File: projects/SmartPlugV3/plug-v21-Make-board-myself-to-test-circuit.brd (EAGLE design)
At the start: 63.5 x 70 mm, 34 parts

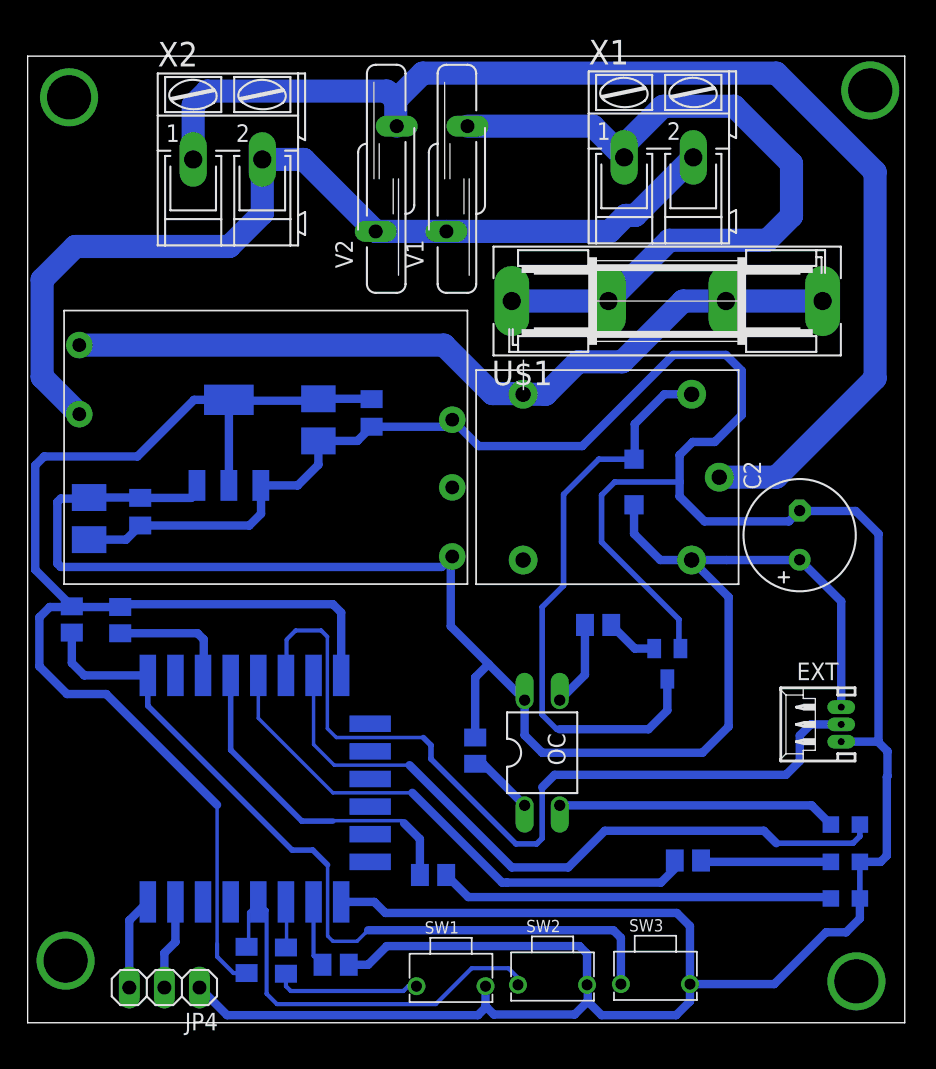
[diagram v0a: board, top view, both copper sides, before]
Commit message: commit message
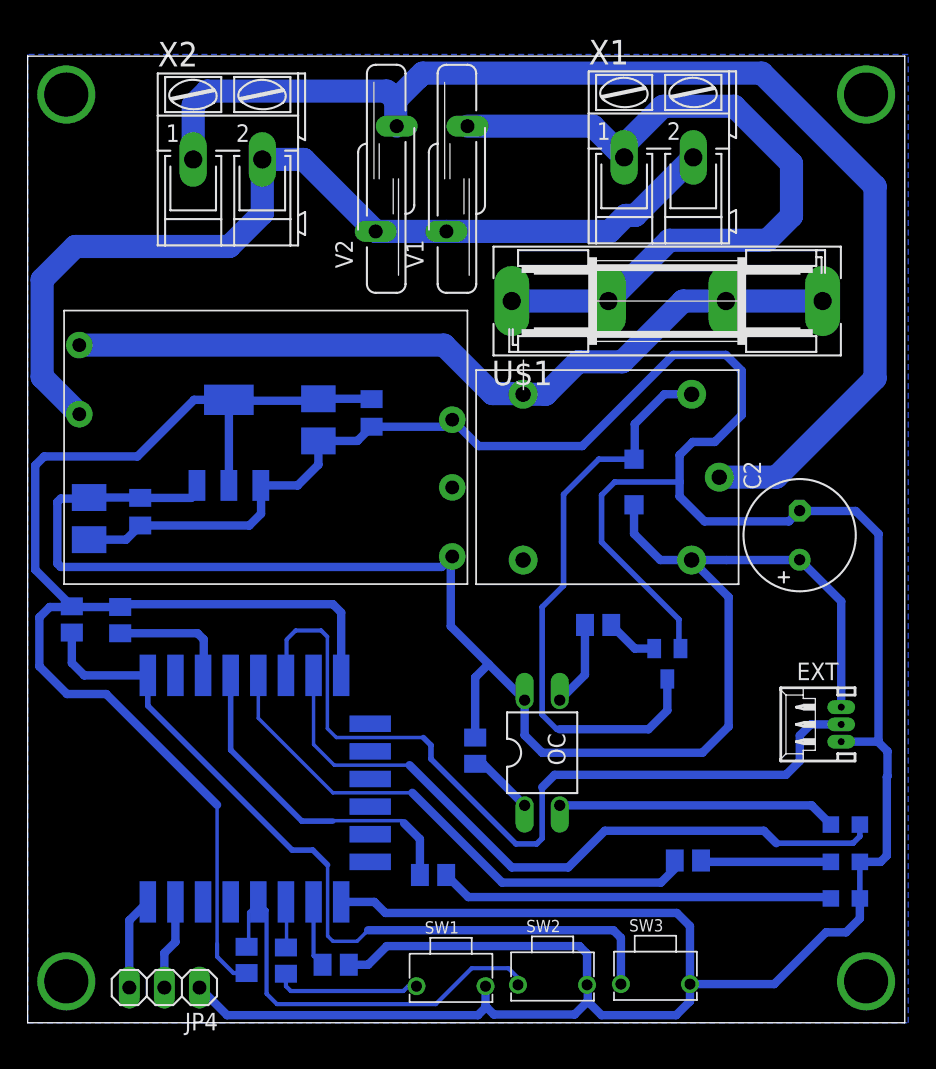
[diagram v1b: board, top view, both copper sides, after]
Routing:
- net RELAY-COM: track 88.9 -> 88.3 mm
- added copper zone on layer 16, net GND
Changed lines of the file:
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@@
 <layer number="37" name="tTest" color="7" fill="1" visible="no" active="yes"/>
 <layer number="38" name="bTest" color="7" fill="1" visible="no" active="yes"/>
-<layer number="39" name="tKeepout" color="4" fill="11" visible="no" active="yes"/>
-<layer number="40" name="bKeepout" color="1" fill="11" visible="no" active="yes"/>
-<layer number="41" name="tRestrict" color="4" fill="10" visible="no" active="yes"/>
-<layer number="42" name="bRestrict" color="1" fill="10" visible="no" active="yes"/>
-<layer number="43" name="vRestrict" color="2" fill="10" visible="no" active="yes"/>
+<layer number="39" name="tKeepout" color="4" fill="11" visible="yes" active="yes"/>
+<layer number="40" name="bKeepout" color="1" fill="11" visible="yes" active="yes"/>
+<layer number="41" name="tRestrict" color="4" fill="10" visible="yes" active="yes"/>
+<layer number="42" name="bRestrict" color="1" fill="10" visible="yes" active="yes"/>
+<layer number="43" name="vRestrict" color="2" fill="10" visible="yes" active="yes"/>
 <layer number="44" name="Drills" color="7" fill="1" visible="no" active="yes"/>
-<layer number="45" name="Holes" color="7" fill="1" visible="no" active="yes"/>
-<layer number="46" name="Milling" color="3" fill="1" visible="no" active="yes"/>
-<layer number="47" name="Measures" color="7" fill="1" visible="no" active="yes"/>
-<layer number="48" name="Document" color="7" fill="1" visible="no" active="yes"/>
-<layer number="49" name="Reference" color="7" fill="1" visible="no" active="yes"/>
+<layer number="45" name="Holes" color="7" fill="1" visible="yes" active="yes"/>
+<layer number="46" name="Milling" color="3" fill="1" visible="yes" active="yes"/>
+<layer number="47" name="Measures" color="7" fill="1" visible="yes" active="yes"/>
+<layer number="48" name="Document" color="7" fill="1" visible="yes" active="yes"/>
+<layer number="49" name="Reference" color="7" fill="1" visible="yes" active="yes"/>
 <layer number="50" name="dxf" color="7" fill="1" visible="no" active="no"/>
-<layer number="51" name="tDocu" color="7" fill="1" visible="no" active="yes"/>
-<layer number="52" name="bDocu" color="7" fill="1" visible="no" active="yes"/>
+<layer number="51" name="tDocu" color="7" fill="1" visible="yes" active="yes"/>
+<layer number="52" name="bDocu" color="7" fill="1" visible="yes" active="yes"/>
 <layer number="53" name="tGND_GNDA" color="7" fill="9" visible="no" active="no"/>
 <layer number="54" name="bGND_GNDA" color="1" fill="9" visible="no" active="no"/>
@@
 <wire x1="62.25" y1="17.85" x2="62.2" y2="17.8" width="0.6096" layer="16"/>
 <wire x1="61.6" y1="20.4" x2="61.55" y2="20.35" width="0.6096" layer="16"/>
+<polygon width="0.4064" layer="16" isolate="0.4064">
+<vertex x="0" y="0"/>
+<vertex x="63.75" y="0"/>
+<vertex x="63.75" y="70.1"/>
+<vertex x="0" y="70.1"/>
+</polygon>
 </signal>
 <signal name="+5V">
@@
 <wire x1="16.7" y1="22.05" x2="22.1" y2="16.65" width="0.254" layer="16"/>
 <wire x1="22.1" y1="16.65" x2="27.85" y2="16.65" width="0.254" layer="16"/>
-<wire x1="34.7" y1="10.15" x2="45.85" y2="10.15" width="0.6096" layer="16"/>
+<wire x1="34.35" y1="10.15" x2="45.85" y2="10.15" width="0.6096" layer="16"/>
 <wire x1="27.85" y1="16.65" x2="34.35" y2="10.15" width="0.6096" layer="16"/>
-<wire x1="34.35" y1="10.15" x2="34.7" y2="10.15" width="0.6096" layer="16"/>
 <wire x1="45.85" y1="10.15" x2="46.85" y2="11.15" width="0.6096" layer="16"/>
 <wire x1="46.85" y1="11.15" x2="46.85" y2="11.75" width="0.4064" layer="16"/>
@@
 <wire x1="26.65" y1="66.8" x2="26.65" y2="64.982" width="1.6764" layer="16"/>
 <wire x1="26.65" y1="64.982" x2="26.722" y2="64.91" width="1.6764" layer="16"/>
-<wire x1="61.35" y1="46.65" x2="61.35" y2="61.6" width="1.6764" layer="16"/>
-<wire x1="61.35" y1="61.6" x2="54.2" y2="68.75" width="1.6764" layer="16"/>
-<wire x1="54.2" y1="68.75" x2="28.6" y2="68.75" width="1.6764" layer="16"/>
-<wire x1="28.6" y1="68.75" x2="26.65" y2="66.8" width="1.6764" layer="16"/>
+<wire x1="28.3" y1="68.45" x2="26.65" y2="66.8" width="1.6764" layer="16"/>
 <wire x1="50.07" y1="39.5" x2="54.2" y2="39.5" width="1.6764" layer="16"/>
 <wire x1="54.2" y1="39.5" x2="61.35" y2="46.65" width="1.6764" layer="16"/>
+<wire x1="61.35" y1="46.65" x2="61.35" y2="60.55" width="1.6764" layer="16"/>
+<wire x1="61.35" y1="60.55" x2="53.15" y2="68.75" width="1.6764" layer="16"/>
+<wire x1="53.15" y1="68.75" x2="28.6" y2="68.75" width="1.6764" layer="16"/>
+<wire x1="28.6" y1="68.75" x2="28.3" y2="68.45" width="1.6764" layer="16"/>
 </signal>
 <signal name="N$6">
@@
 </signal>
 <signal name="N$3">
-<via x="3" y="67" extent="1-16" drill="3.2"/>
+<via x="2.8" y="67.2" extent="1-16" drill="3.2"/>
 </signal>
 <signal name="N$4">
-<via x="2.75" y="4.5" extent="1-16" drill="3.2"/>
+<via x="2.8" y="3" extent="1-16" drill="3.2"/>
 </signal>
 <signal name="N$5">
-<via x="60" y="3" extent="1-16" drill="3.2"/>
+<via x="60.7" y="3" extent="1-16" drill="3.2"/>
 </signal>
 <signal name="N$7">
-<via x="61" y="67.5" extent="1-16" drill="3.2"/>
+<via x="60.7" y="67.2" extent="1-16" drill="3.2"/>
 </signal>
 <signal name="G-02">
